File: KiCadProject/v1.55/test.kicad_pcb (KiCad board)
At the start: 2 copper layers, 88.9 x 67.3 mm, 24 parts, among them J1 CONN_01X01_MALE, J2 MY_USB_OTG, SW1 SW_DIP_x02, SW2 SW_DIP_x02, U1 TinyRTC_I2C_RIGHT, U2 MAX7219_IN, U3 MAX7219_IN, U4 MAX7219_IN, U5 MAX7219_IN, U6 MAX7219_IN, U7 MAX7219_IN, U8 ATMEGA328P-PU, U9 FTDI1232, Y1 Crystal

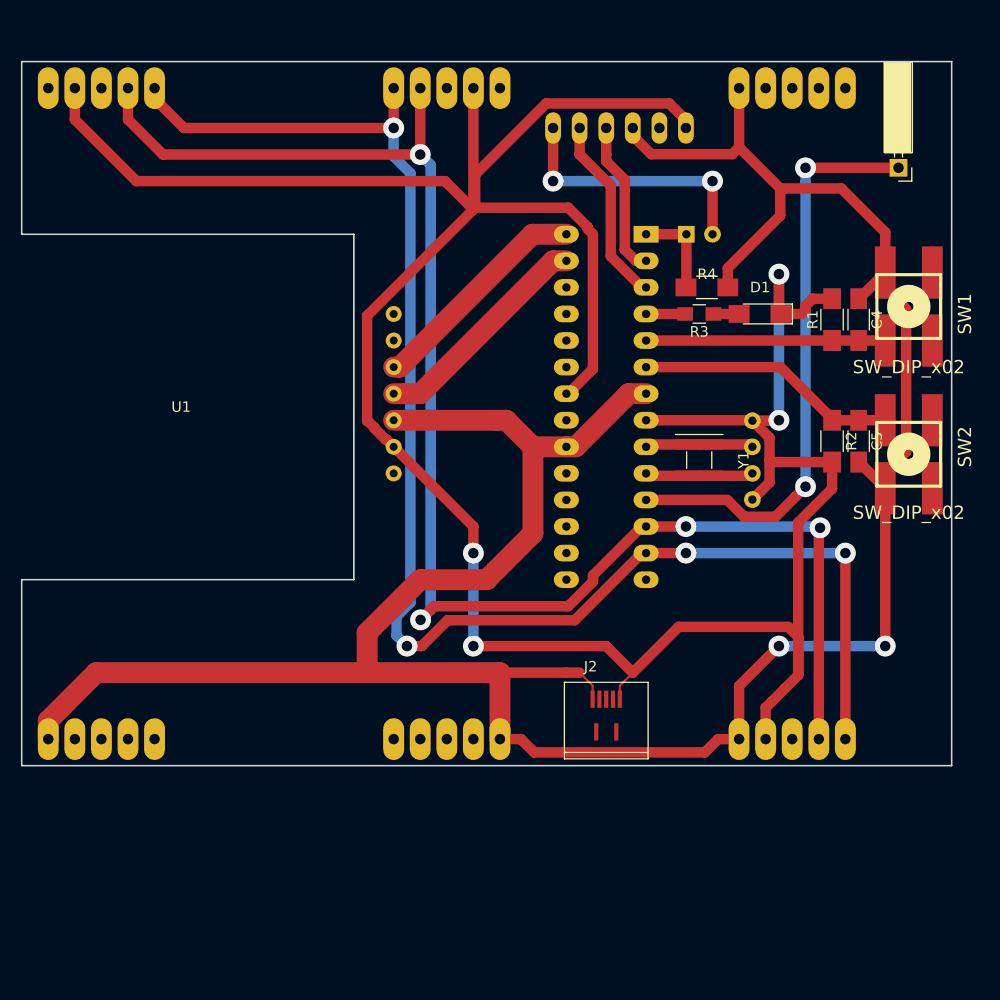
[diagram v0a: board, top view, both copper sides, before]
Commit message: v1.55
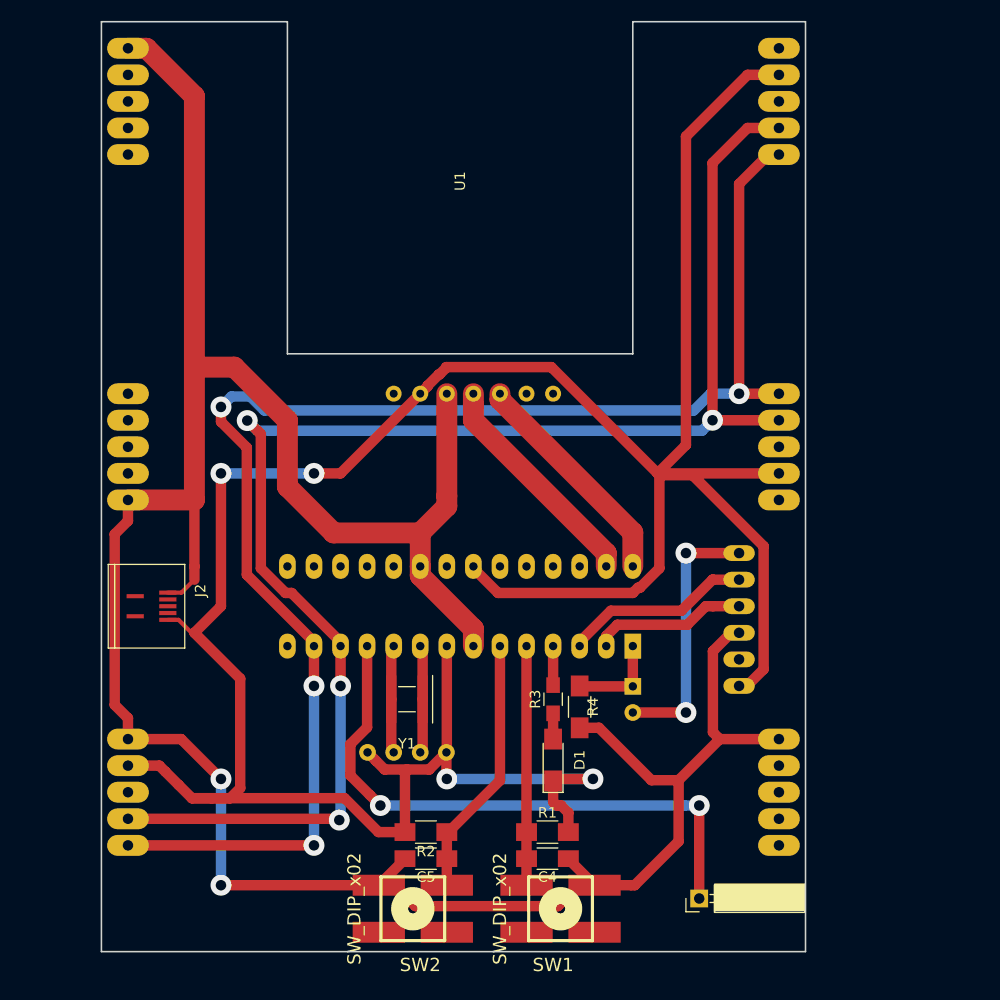
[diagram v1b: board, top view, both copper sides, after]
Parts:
- moved J1 72.4 mm to (166.4, 130.8), turned to 180 degrees
- moved U5 70.0 mm to (174.0, 49.5), turned to 180 degrees
- moved SW1 66.5 mm to (153.1, 131.8), turned to 270 degrees
- moved U2 66.5 mm to (111.8, 49.5), turned to 180 degrees
- moved SW2 64.3 mm to (139.0, 131.8), turned to 270 degrees
- moved U7 62.3 mm to (174.0, 115.6), turned to 180 degrees
- moved C4 59.5 mm to (151.9, 127.0), turned to 180 degrees
- moved U4 58.4 mm to (111.8, 115.6), turned to 180 degrees
- moved C5 57.5 mm to (140.2, 127.0), turned to 180 degrees
- moved R1 56.0 mm to (151.9, 124.5), turned to 0 degrees
- moved R2 53.9 mm to (140.2, 124.5), turned to 180 degrees
- moved U6 47.6 mm to (174.0, 92.7), turned to 0 degrees
- moved D1 47.0 mm to (152.4, 117.6), turned to 90 degrees
- moved J2 44.6 mm to (114.1, 102.9), turned to 270 degrees
- moved U9 44.4 mm to (170.2, 97.8), turned to 270 degrees
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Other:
- board size 88.9 x 67.3 mm -> 67.3 x 88.9 mm
- net class 0,4mm: clearance 0.1 -> 0.2
